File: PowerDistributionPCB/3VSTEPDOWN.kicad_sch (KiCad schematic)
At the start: 8 parts

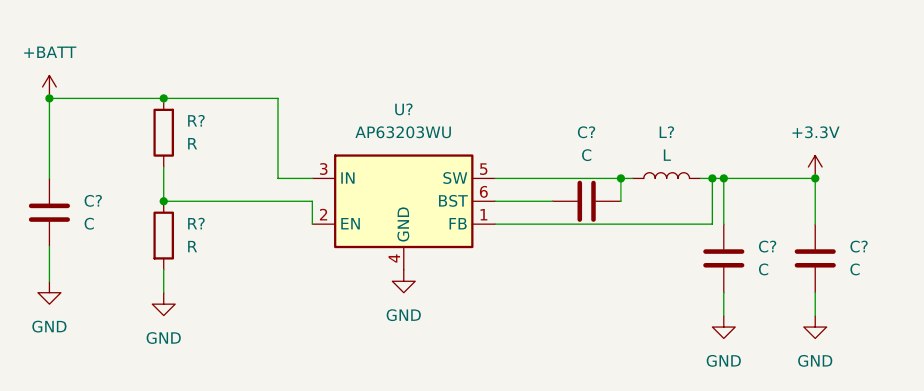
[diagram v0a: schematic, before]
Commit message: updated 3.3V stepdown
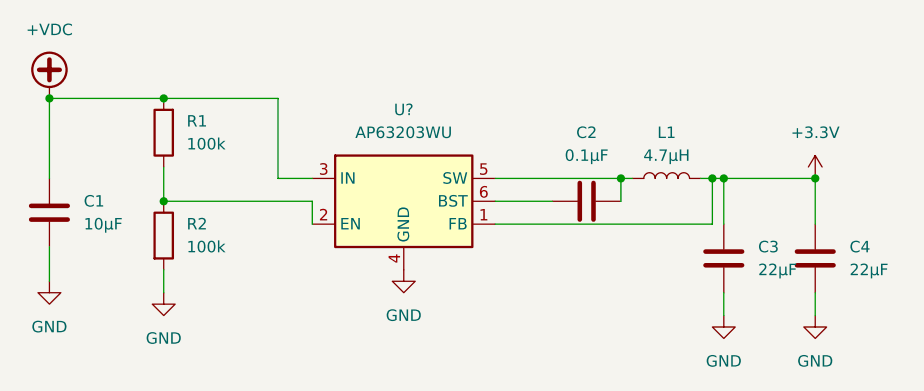
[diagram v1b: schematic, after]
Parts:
- C1: renamed from C?; value C -> 10µF
- C2: renamed from C?; value C -> 0.1µF
- C3, C4: renamed from C?; value C -> 22µF
- L1: renamed from L?; value L -> 4.7µH
- R1, R2: renamed from R?; value R -> 100k
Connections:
- net +BATT renamed +VDC

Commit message: relay implementation
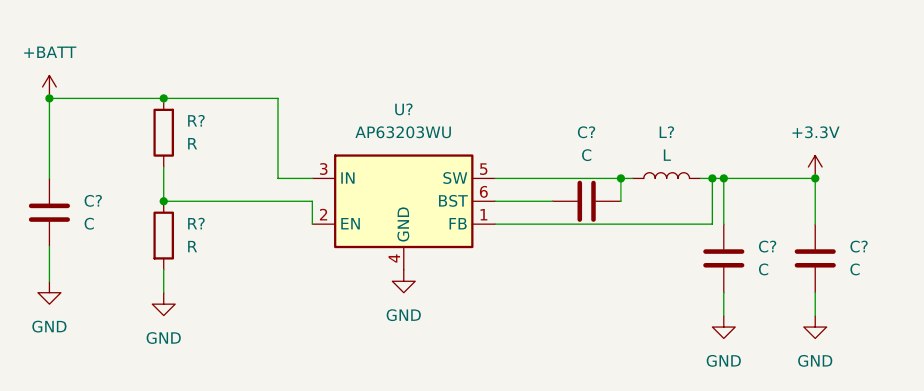
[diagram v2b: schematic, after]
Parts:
- C?: renamed from C4; value 22µF -> C
- C?: renamed from C1; value 10µF -> C
- C?: renamed from C2; value 0.1µF -> C
- C?: renamed from C3; value 22µF -> C
- L?: renamed from L1; value 4.7µH -> L
- R?: renamed from R2; value 100k -> R
- R?: renamed from R1; value 100k -> R
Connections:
- net +VDC renamed +BATT
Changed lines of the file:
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@@
+	)
+	(junction
+		(at 104.14 68.58)
+		(diameter 0)
+		(color 0 0 0 0)
 	)
 	(junction
@@
 	)
 	(junction
-		(at 104.14 68.58)
-		(diameter 0)
-		(color 0 0 0 0)
-	)
-	(junction
 		(at 116.84 68.58)
 		(diameter 0)
@@
 	)
 	(symbol
+		(lib_id "power:+BATT")
+		(at 104.14 68.58 0)
+		(unit 1)
+		(exclude_from_sim no)
+		(in_bom yes)
+		(on_board yes)
+		(dnp no)
+		(fields_autoplaced yes)
+		(property "Reference" "#PWR020"
+			(at 104.14 72.39 0)
+			(effects
+				(font
+					(size 1.27 1.27)
+				)
+				(hide yes)
+			)
+		)
+		(property "Value" "+BATT"
+			(at 104.14 63.5 0)
+			(effects
+				(font
+					(size 1.27 1.27)
+				)
+			)
+		)
+		(property "Footprint" ""
+			(at 104.14 68.58 0)
+			(effects
+				(font
+					(size 1.27 1.27)
+				)
+				(hide yes)
+			)
+		)
+		(property "Datasheet" ""
+			(at 104.14 68.58 0)
+			(effects
+				(font
+					(size 1.27 1.27)
+				)
+				(hide yes)
+			)
+		)
+		(property "Description" "Power symbol creates a global label with name \"+BATT\""
+			(at 104.14 68.58 0)
+			(effects
+				(font
+					(size 1.27 1.27)
+				)
+				(hide yes)
+			)
+		)
+		(pin "1"
+		)
+		(instances
+			(project ""
+				(path "/b27c75df-6223-4cc6-be69-062c2b02d5c6/079a49e6-596e-4e19-9f4e-bda307b8342c"
+					(reference "#PWR020")
+					(unit 1)
+				)
+			)
+		)
+	)
+	(symbol
 		(lib_id "Regulator_Switching:AP63203WU")
 		(at 143.51 80.01 0)
@@
 		(dnp no)
 		(fields_autoplaced yes)
-		(property "Reference" "R2"
+		(property "Reference" "R?"
 			(at 119.38 82.5499 0)
 			(effects
@@
 			)
 		)
-		(property "Value" "100k"
+		(property "Value" "R"
 			(at 119.38 85.0899 0)
 			(effects
@@
 			(project ""
 				(path "/b27c75df-6223-4cc6-be69-062c2b02d5c6/079a49e6-596e-4e19-9f4e-bda307b8342c"
-					(reference "R2")
+					(reference "R?")
 					(unit 1)
 				)
@@
 		(dnp no)
 		(fields_autoplaced yes)
-		(property "Reference" "C4"
+		(property "Reference" "C?"
 			(at 193.04 85.0899 0)
 			(effects
@@
 			)
 		)
-		(property "Value" "22µF"
+		(property "Value" "C"
 			(at 193.04 87.6299 0)
 			(effects
@@
 			(project ""
 				(path "/b27c75df-6223-4cc6-be69-062c2b02d5c6/079a49e6-596e-4e19-9f4e-bda307b8342c"
-					(reference "C4")
+					(reference "C?")
 					(unit 1)
 				)
@@
 		(dnp no)
 		(fields_autoplaced yes)
-		(property "Reference" "R1"
+		(property "Reference" "R?"
 			(at 119.38 71.1199 0)
 			(effects
@@
 			)
 		)
-		(property "Value" "100k"
+		(property "Value" "R"
 			(at 119.38 73.6599 0)
 			(effects
@@
 			(project ""
 				(path "/b27c75df-6223-4cc6-be69-062c2b02d5c6/079a49e6-596e-4e19-9f4e-bda307b8342c"
-					(reference "R1")
+					(reference "R?")
 					(unit 1)
 				)
@@
 		(dnp no)
 		(fields_autoplaced yes)
-		(property "Reference" "C1"
+		(property "Reference" "C?"
 			(at 107.95 80.0099 0)
 			(effects
@@
 			)
 		)
-		(property "Value" "10µF"
+		(property "Value" "C"
 			(at 107.95 82.5499 0)
 			(effects
@@
 			(project ""
 				(path "/b27c75df-6223-4cc6-be69-062c2b02d5c6/079a49e6-596e-4e19-9f4e-bda307b8342c"
-					(reference "C1")
+					(reference "C?")
 					(unit 1)
 				)
@@
 		(dnp no)
 		(fields_autoplaced yes)
-		(property "Reference" "C2"
+		(property "Reference" "C?"
 			(at 163.83 72.39 90)
 			(effects
@@
 			)
 		)
-		(property "Value" "0.1µF"
+		(property "Value" "C"
 			(at 163.83 74.93 90)
 			(effects
@@
 			(project ""
 				(path "/b27c75df-6223-4cc6-be69-062c2b02d5c6/079a49e6-596e-4e19-9f4e-bda307b8342c"
-					(reference "C2")
+					(reference "C?")
 					(unit 1)
 				)
@@
 		(dnp no)
 		(fields_autoplaced yes)
-		(property "Reference" "C3"
+		(property "Reference" "C?"
 			(at 182.88 85.0899 0)
 			(effects
@@
 			)
 		)
-		(property "Value" "22µF"
+		(property "Value" "C"
 			(at 182.88 87.6299 0)
 			(effects
@@
 			(project ""
 				(path "/b27c75df-6223-4cc6-be69-062c2b02d5c6/079a49e6-596e-4e19-9f4e-bda307b8342c"
-					(reference "C3")
+					(reference "C?")
 					(unit 1)
 				)
@@
 	)
 	(symbol
-		(lib_id "power:+VDC")
-		(at 104.14 68.58 0)
-		(unit 1)
-		(exclude_from_sim no)
-		(in_bom yes)
-		(on_board yes)
-		(dnp no)
-		(fields_autoplaced yes)
-		(property "Reference" "#PWR020"
-			(at 104.14 71.12 0)
-			(effects
-				(font
-					(size 1.27 1.27)
-				)
-				(hide yes)
-			)
-		)
-		(property "Value" "+VDC"
-			(at 104.14 60.96 0)
-			(effects
-				(font
-					(size 1.27 1.27)
-				)
-			)
-		)
-		(property "Footprint" ""
-			(at 104.14 68.58 0)
-			(effects
-				(font
-					(size 1.27 1.27)
-				)
-				(hide yes)
-			)
-		)
-		(property "Datasheet" ""
-			(at 104.14 68.58 0)
-			(effects
-				(font
-					(size 1.27 1.27)
-				)
-				(hide yes)
-			)
-		)
-		(property "Description" "Power symbol creates a global label with name \"+VDC\""
-			(at 104.14 68.58 0)
-			(effects
-				(font
-					(size 1.27 1.27)
-				)
-				(hide yes)
-			)
-		)
-		(pin "1"
-		)
-		(instances
-			(project ""
-				(path "/b27c75df-6223-4cc6-be69-062c2b02d5c6/079a49e6-596e-4e19-9f4e-bda307b8342c"
-					(reference "#PWR020")
-					(unit 1)
-				)
-			)
-		)
-	)
-	(symbol
 		(lib_id "power:GND")
 		(at 189.23 92.71 0)
@@
 		(dnp no)
 		(fields_autoplaced yes)
-		(property "Reference" "L1"
+		(property "Reference" "L?"
 			(at 172.72 72.39 90)
 			(effects
@@
 			)
 		)
-		(property "Value" "4.7µH"
+		(property "Value" "L"
 			(at 172.72 74.93 90)
 			(effects
@@
 			(project ""
 				(path "/b27c75df-6223-4cc6-be69-062c2b02d5c6/079a49e6-596e-4e19-9f4e-bda307b8342c"
-					(reference "L1")
-					(unit 1)
-				)
+					(reference "L?")
+					(unit 1)
+				)
